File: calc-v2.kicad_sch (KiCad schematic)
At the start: 110 parts, among them IC1 ISL91107IRTNZ-T, J1 USB_C_Receptacle_USB2.0_16P, J2 Conn_01x02_MountingPin, SW1 SW_Push_45deg, SW10 SW_Push_45deg, SW11 SW_Push_45deg, SW12 SW_Push_45deg, SW13 SW_Push_45deg, SW14 SW_Push_45deg, SW15 SW_Push_45deg, SW16 SW_Push_45deg, SW17 SW_Push_45deg, SW18 SW_Push_45deg, SW19 SW_Push_45deg, SW2 SW_Push_45deg, SW20 SW_Push_45deg, SW21 SW_Push_45deg, SW22 SW_Push_45deg, SW23 SW_Push_45deg, SW24 SW_Push_45deg, SW25 SW_Push_45deg, SW26 SW_Push_45deg, SW27 SW_Push_45deg, SW28 SW_Push_45deg, SW29 SW_Push_45deg, SW3 SW_Push_45deg, SW30 SW_Push_45deg, SW31 SW_Push_45deg, SW32 SW_Push_45deg, SW33 SW_Push_45deg, SW34 SW_Push_45deg, SW35 SW_Push_45deg, SW36 SW_Push_45deg, SW37 SW_Push_45deg, SW38 SW_Push_45deg, SW39 SW_Push_45deg, SW4 SW_Push_45deg, SW40 SW_Push_45deg, SW41 SW_Push_45deg, SW42 SW_Push_45deg, SW43 SW_Push_45deg, SW44 SW_Push_45deg, SW45 SW_Push_45deg, SW46 SW_Push_45deg, SW47 SW_Push_45deg, SW48 SW_Push_45deg, SW49 SW_Push_45deg, SW5 SW_Push_45deg, SW6 SW_Push_45deg, SW7 SW_Push_45deg, SW8 SW_Push_45deg, SW9 SW_Push_45deg, U1 W25Q128JVS, U3 BQ24074RGT, U4 TPS61165DBV, U5 RP2350B, U6 APS6404L-3SQRx-ZR, Y1 ABM8-272-T3

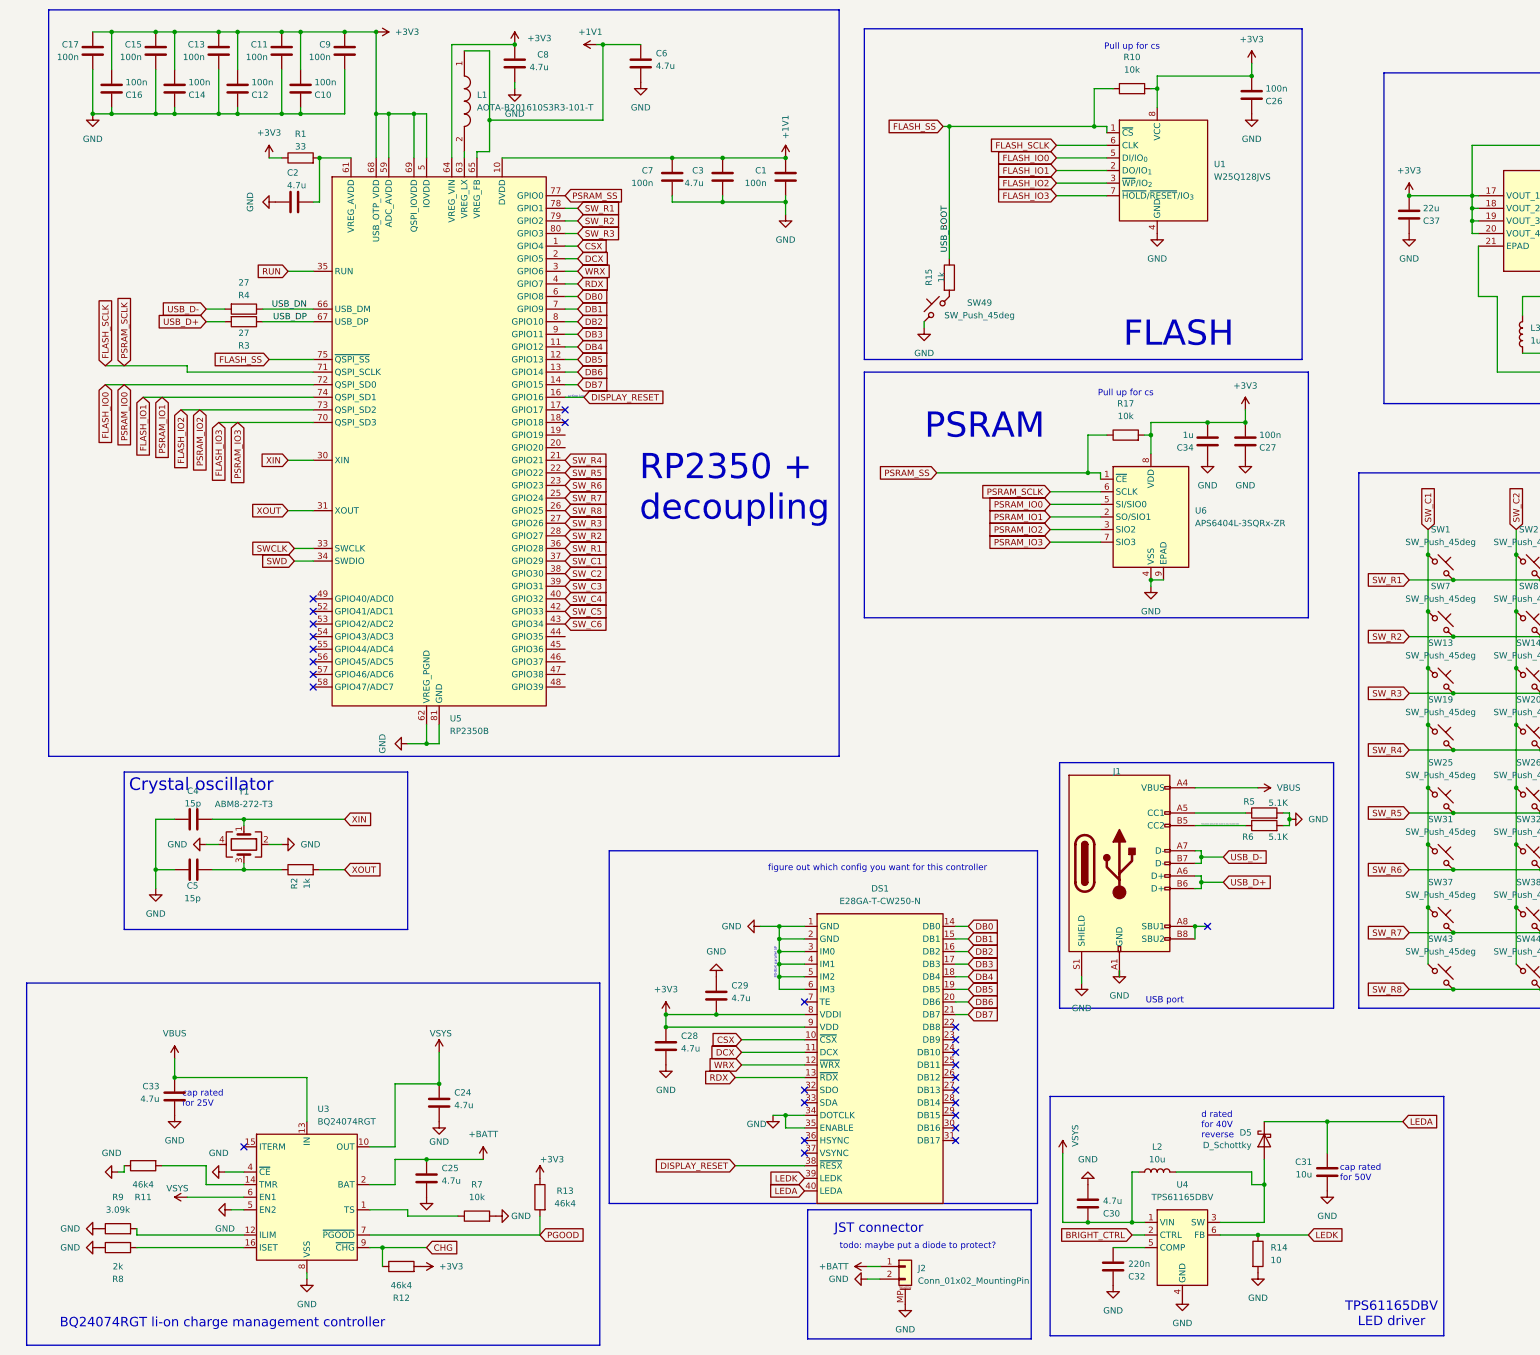
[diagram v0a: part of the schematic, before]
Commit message: various things
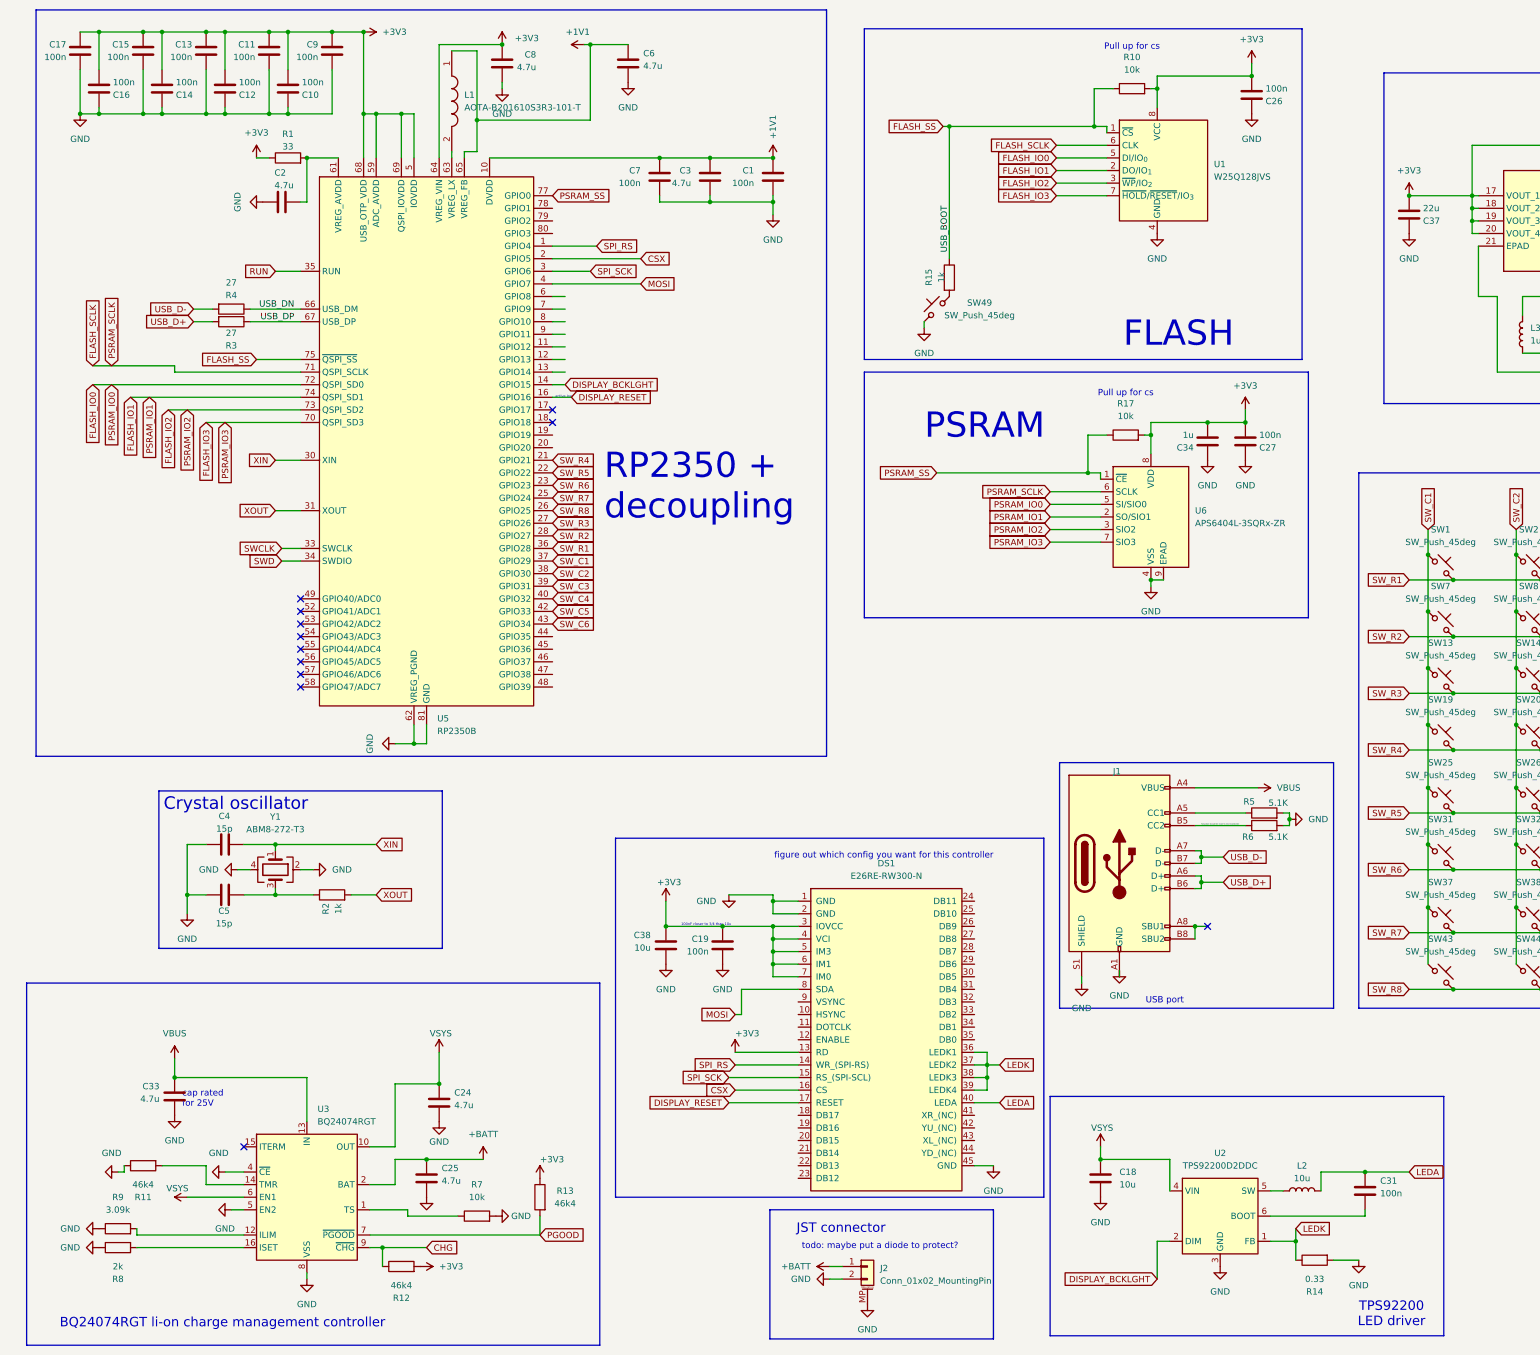
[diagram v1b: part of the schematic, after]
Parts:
- removed C28, C29, C30: 4.7u, Capacitor_SMD:C_0402_1005Metric, symbol Device:C
- removed C32: 220n, Capacitor_SMD:C_0402_1005Metric, symbol Device:C
- removed D5: D_Schottky, Diode_SMD:D_0402_1005Metric, symbol Device:D_Schottky
- removed DS1: E28GA-T-CW250-N, AAAAA:HIROSE_FH12S-40S-0.5SH_55_, symbol AAAAAAA:E28GA-T-CW250-N
- removed U4: TPS61165DBV, Package_TO_SOT_SMD:SOT-23-6, symbol Driver_LED:TPS61165DBV
- added C18, C38: 10u, Capacitor_SMD:C_0402_1005Metric, symbol Device:C
- added C19: 100n, Capacitor_SMD:C_0402_1005Metric, symbol Device:C
- added DS1: E26RE-RW300-N, AAAAA:HRS_FH12-45S-0.5SH_55_, symbol AAAAAAA:E26RE-RW300-N
- added U2: TPS92200D2DDC, Package_TO_SOT_SMD:SOT-23-6, symbol Driver_LED:TPS92200D2DDC
- C1, C17, C3, C7: footprint (none) -> Capacitor_SMD:C_0402_1005Metric
- C31: value 10u -> 100n
- J1: footprint (none) -> Connector_USB:USB_C_Receptacle_Amphenol_124019772112A
- L2, L3: footprint (none) -> Inductor_SMD:L_0201_0603Metric
- R1, R10, R11, R12, R13, R17, R3, R4, R5, R6, R7, R8, R9: footprint (none) -> Resistor_SMD:R_0201_0603Metric
- R14: value 10 -> 0.33; footprint (none) -> Resistor_SMD:R_0201_0603Metric
- Y1: footprint ABM8-272-T3:XTAL_ABM8-272-T3 -> AAAAA:ABM8272T3
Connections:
- net DCX is gone; now on net CSX: U5.2 (GPIO5)
- net +3V3: now also C19.1, C38.1, DS1.13 (RD), DS1.3 (IOVCC), DS1.4 (VCI), DS1.5 (IM3), DS1.6 (IM1), DS1.7 (IM0)
- net CSX: now also DS1.16 (CS); no longer U5.1 (GPIO4)
- net DISPLAY_RESET: now also DS1.17 (RESET)
- net GND: now also C18.2, C19.2, C38.2, DS1.1 (GND), DS1.2 (GND), DS1.45 (GND), U2.3 (GND); no longer C31.2
- net LEDA: now also L2.2, DS1.40 (LEDA)
- net LEDK: now also DS1.36 (LEDK1), DS1.37 (LEDK2), DS1.38 (LEDK3), DS1.39 (LEDK4), U2.1 (FB)
- net SW_R1: no longer U5.78 (GPIO1)
- net SW_R2: no longer U5.79 (GPIO2)
- net SW_R3: no longer U5.80 (GPIO3)
- net VSYS: now also C18.1, U2.4 (VIN); no longer L2.1
- net DB0: no longer names the net of U5.6 (GPIO8)
- net DB1: no longer names the net of U5.7 (GPIO9)
- net DB2: no longer names the net of U5.8 (GPIO10)
- net DB3: no longer names the net of U5.9 (GPIO11)
- net DB4: no longer names the net of U5.11 (GPIO12)
- net DB5: no longer names the net of U5.12 (GPIO13)
- net DB6: no longer names the net of U5.13 (GPIO14)
- net DB7 renamed DISPLAY_BCKLGHT
- net DISPLAY_BCKLGHT: now also U2.2 (DIM)
- net RDX renamed MOSI
- net MOSI: now also DS1.8 (SDA)
- net WRX renamed SPI_SCK
- net SPI_SCK: now also DS1.15 (RS_(SPI-SCL))
- new net: L2.1, U2.5 (SW)
- new net: C31.2, U2.6 (BOOT)
- new net SPI_RS: DS1.14 (WR_(SPI-RS)), U5.1 (GPIO4)
- no-connect marks 29 -> 14
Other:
- note added: "100nF closer to 3/4 than 10u"
- note added: "TPS92200 LED driver"
- note removed: "80-8bit parallel I/F"
- note removed: "TPS61165DBV LED driver"
- note removed: "cap rated for 50V"
- note removed: "d rated for 40V reverse"
- moved on the sheet: C1, C10, C11, C12, C13, C14, C15, C16, C17, C2, C3, C4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
